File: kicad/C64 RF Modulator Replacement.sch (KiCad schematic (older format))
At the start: 33 parts, among them J1 Conn_01x04_Male, J2 Conn_01x04_Male, Q1 BC547, Q2 BC547, U1 78L05

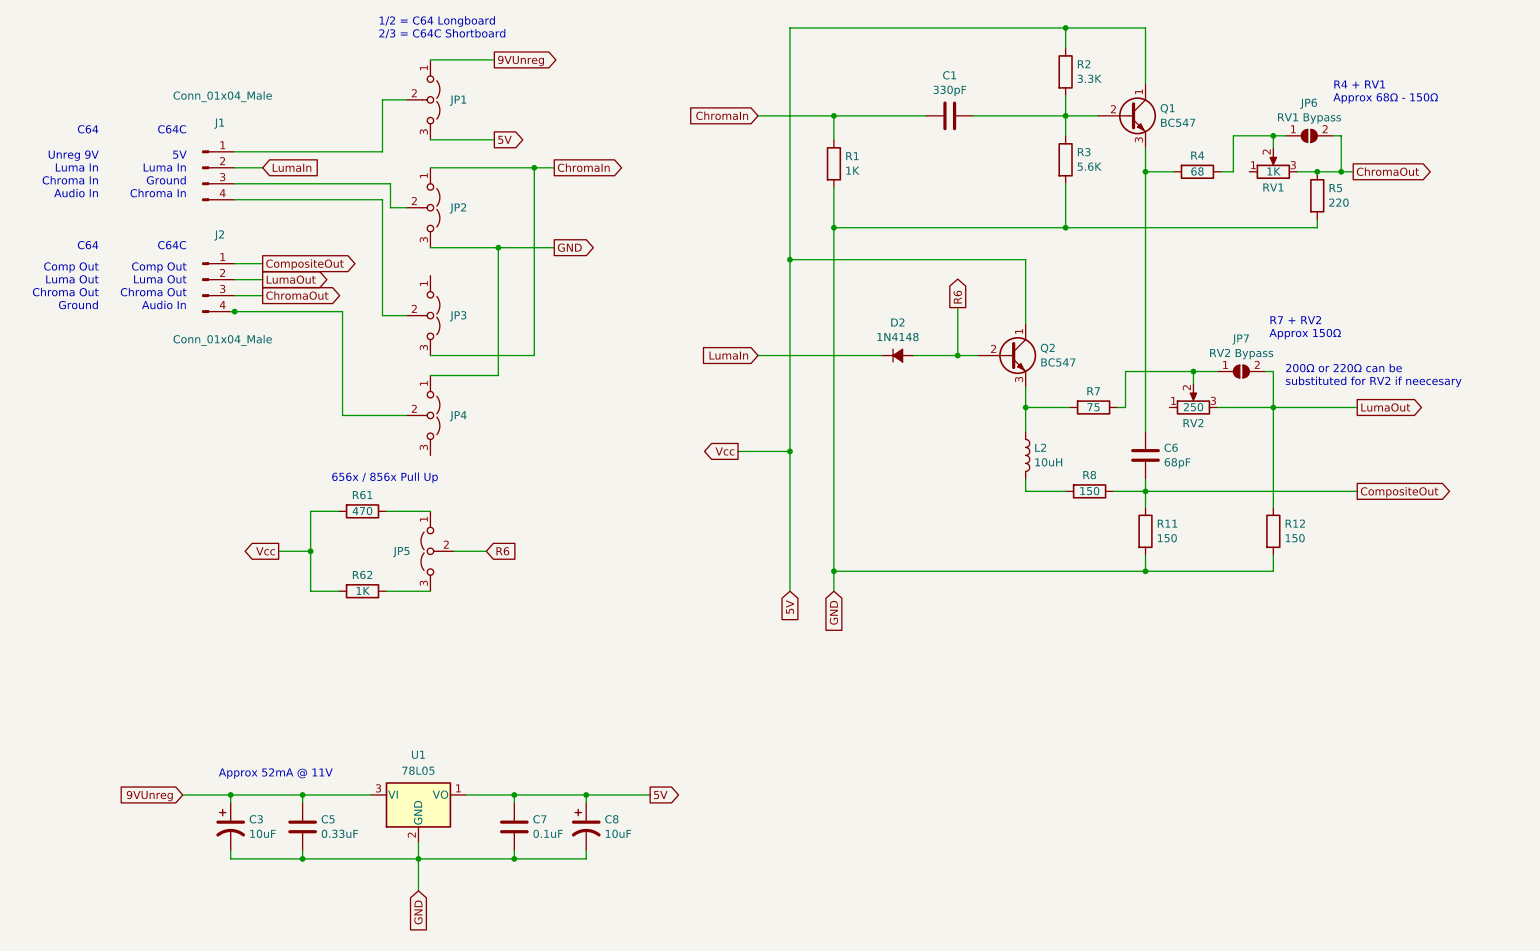
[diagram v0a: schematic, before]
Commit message: Rev C
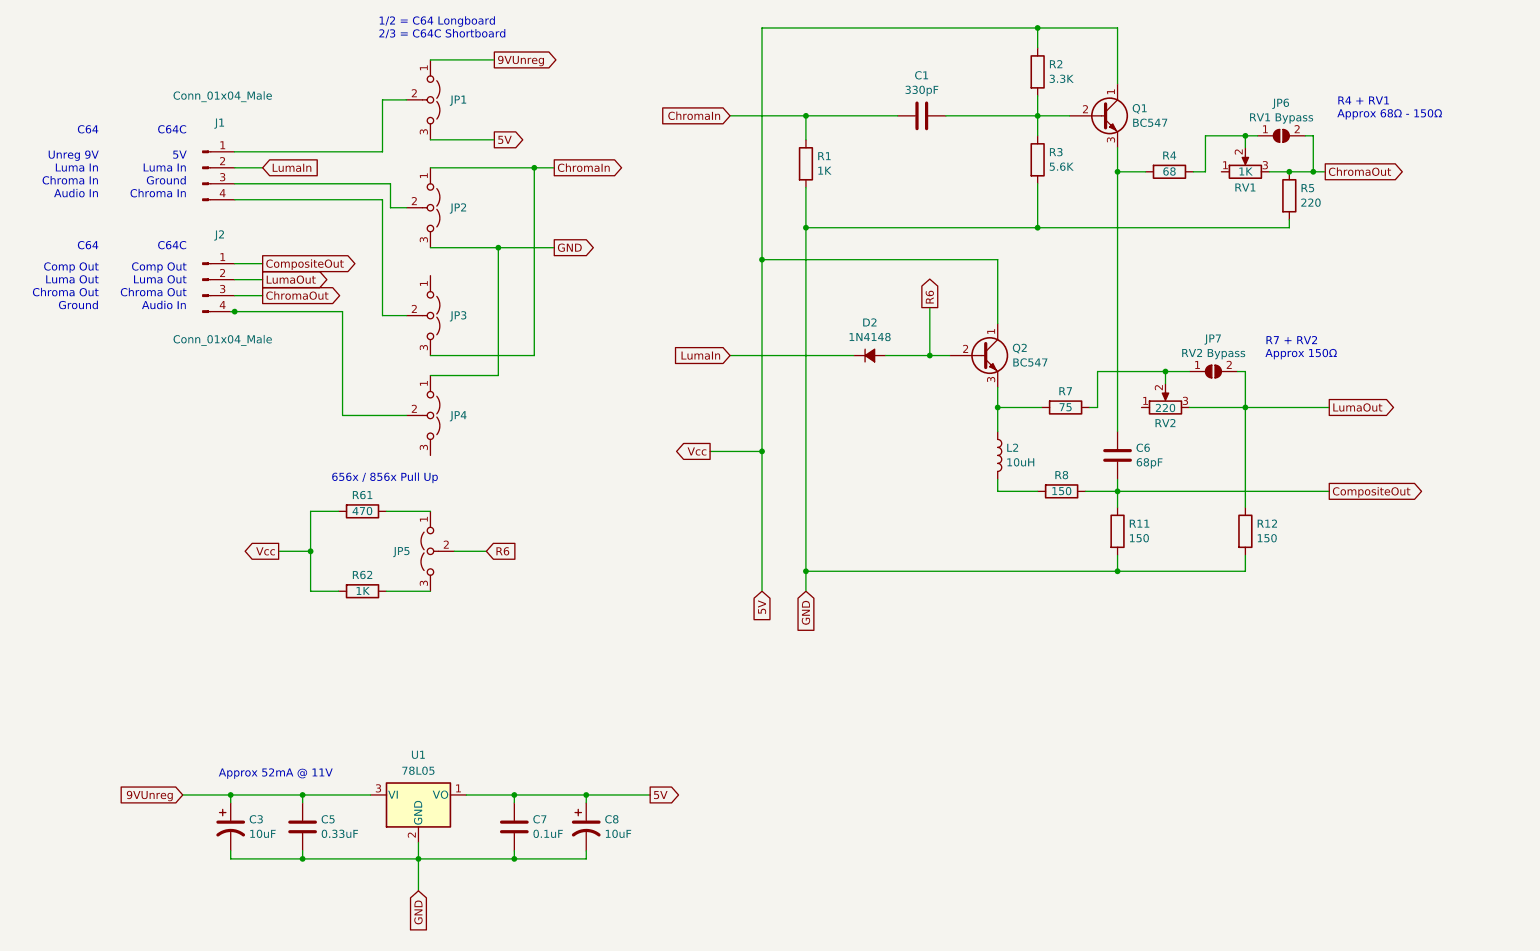
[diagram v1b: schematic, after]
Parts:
- RV1: footprint Potentiometer_THT:Potentiometer_Bourns_3296Y_Vertical -> Potentiometer_THT:Potentiometer_Bourns_3296W_Vertical
- RV2: value 250 -> 220; footprint Potentiometer_THT:Potentiometer_Bourns_3296Y_Vertical -> Potentiometer_THT:Potentiometer_Bourns_3296W_Vertical
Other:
- note removed: "200Ω or 220Ω can be \nsubstituted for RV2 if neecesary"
- moved on the sheet: C1, C6, D2, JP6, JP7, L2, Q1, Q2, R1, R11, R12, R2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
